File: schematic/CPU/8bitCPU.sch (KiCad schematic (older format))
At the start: 28 parts, among them U29 74LS08, U77 74LS245

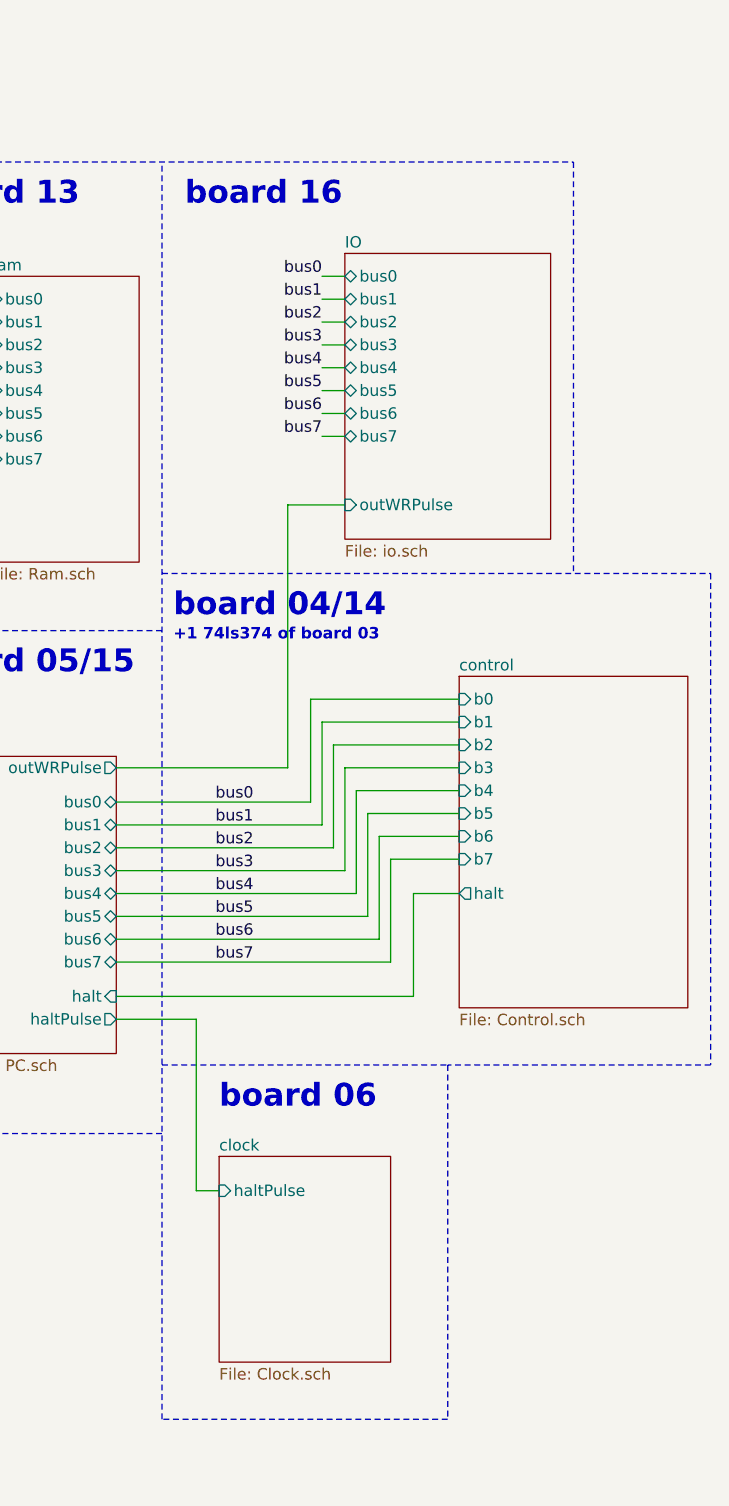
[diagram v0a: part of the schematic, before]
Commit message: updated schematic
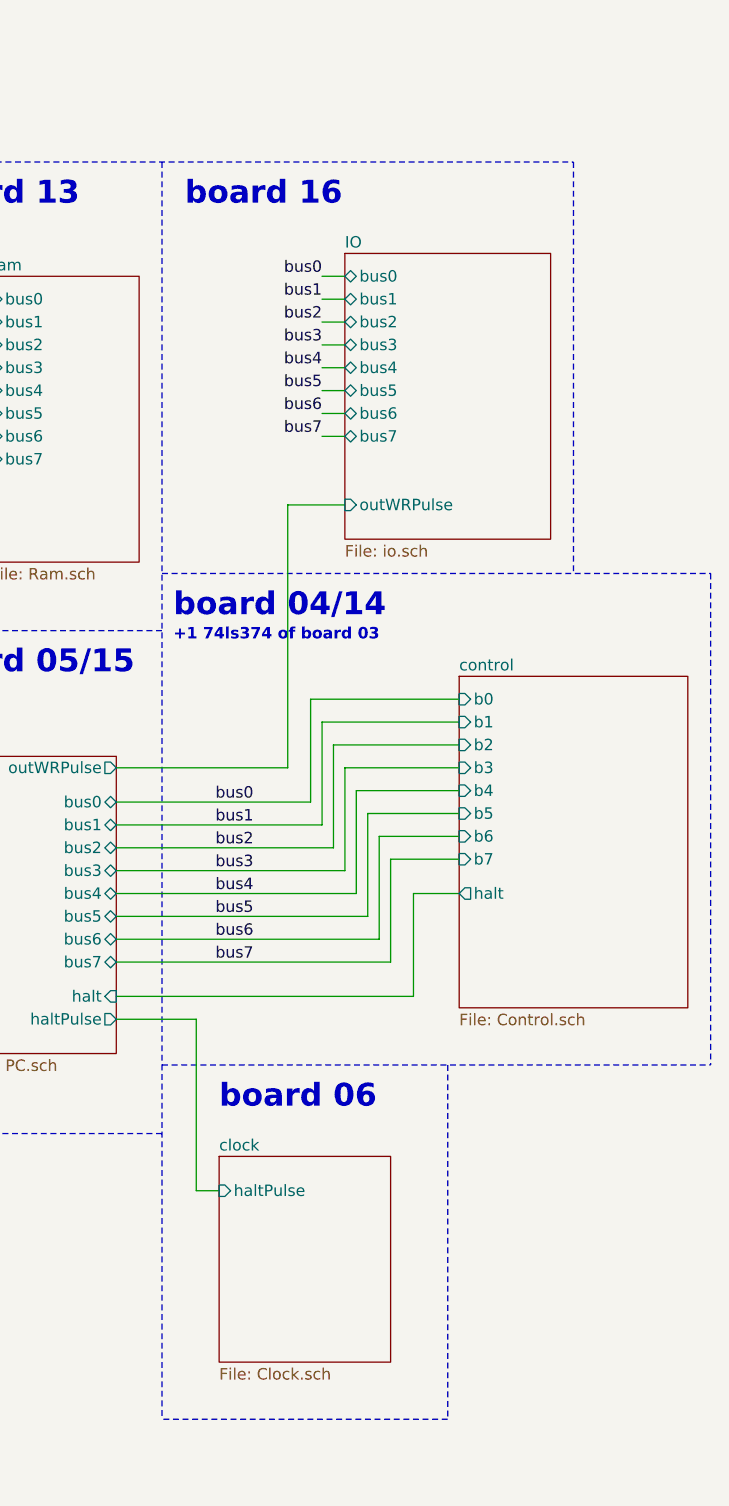
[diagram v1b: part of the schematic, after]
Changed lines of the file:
@@
 F8 "b6" I L 12600 5050 50
 F9 "b7" I L 12600 5150 50
-F11 "halt" O L 12600 5300 50
+F10 "halt" O L 12600 5300 50
 $EndSheet
 Text Label 11700 4900 2    50   ~ 0
@@
 	2300 2100 13100 2100
 Wire Notes Line width 12
-	11300 7350 11300 2100
-Wire Notes Line width 12
 	12550 6050 12550 7600
 Wire Notes Line width 12
 	13700 3900 13700 6050
-Wire Notes Line width 12
-	13700 6050 12550 6050
 Text Notes 11350 4100 0    100  ~ 20
 board 04/14
@@
 	11300 3900 13700 3900
 Wire Notes Line width 12
-	11300 6050 12550 6050
-Wire Notes Line width 12
 	12550 7600 11300 7600
-Wire Notes Line width 12
-	11300 7600 11300 7350
 Text Notes 11350 4200 0    50   ~ 10
 +1 74ls374 of board 03
+Wire Notes Line width 12
+	11300 2100 11300 7600
+Wire Notes Line width 12
+	11300 6050 13700 6050
 $EndSCHEMATC
